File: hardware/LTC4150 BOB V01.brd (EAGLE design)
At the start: 21 parts, among them U1 LTC4150

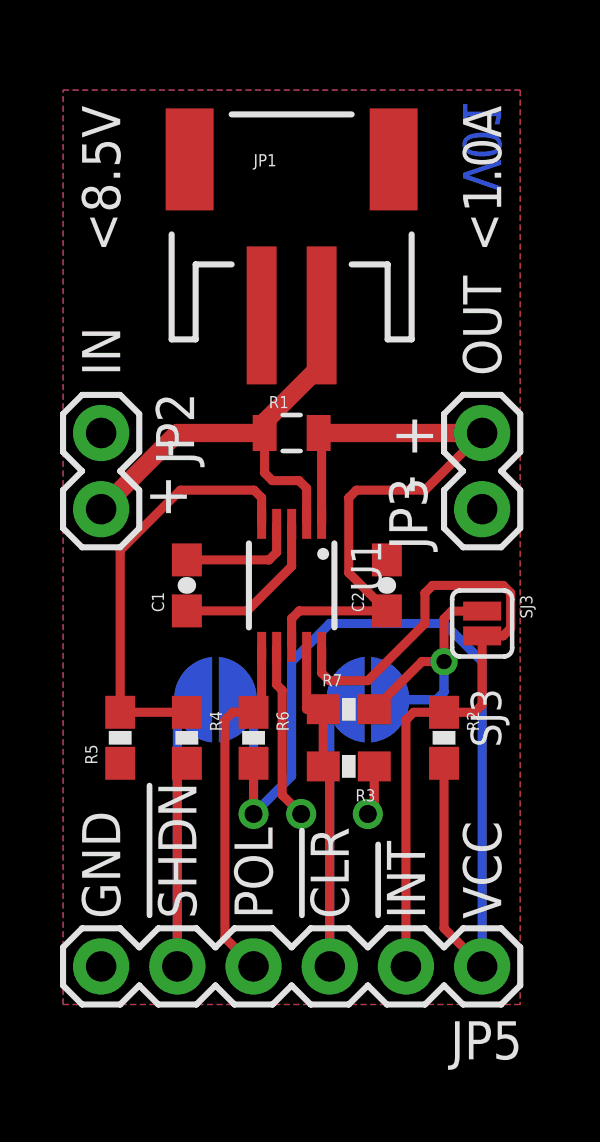
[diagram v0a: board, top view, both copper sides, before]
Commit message: Ready for proto?
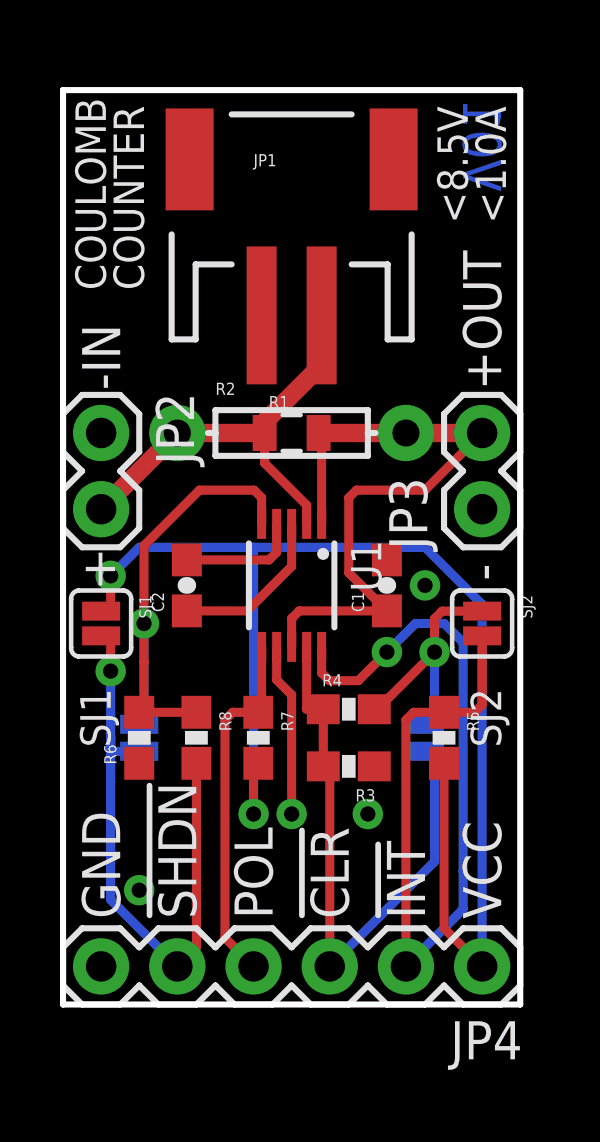
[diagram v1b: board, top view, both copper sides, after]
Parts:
- added R8: 75K, SparkFun-Passives:0603-RES
- added SJ4: (no value), mike-temp:SJ_2S-NO
- LOGO1: value LOGO-SFESK -> OSHW-LOGOS; device SparkFun-Aesthetics:SFE-LOGO-FLAME -> SparkFun-Aesthetics:OSHW-LOGO-S
- LOGO2: value OSHW-LOGOS -> LOGO-SFENW2; device SparkFun-Aesthetics:OSHW-LOGO-S -> SparkFun-Aesthetics:SFE-NEW-WEB
- LOGO3: value LOGO-SFENW2 -> LOGO-SFESK; device SparkFun-Aesthetics:SFE-NEW-WEB -> SparkFun-Aesthetics:SFE-LOGO-FLAME
- R2: value 3K -> DNP; device SparkFun-Passives:0603-RES -> SparkFun-Passives:AXIAL-0.3
- R5, R7: value 75K -> 3K
- R6: value 3K -> 75K
- SJ1: device mike-temp:SJ_ROUND -> mike-temp:SJ_2S
- SJ2: device mike-temp:SJ_ROUND -> SparkFun-Passives:SJ_2S
- SJ3: device SparkFun-Passives:SJ_2S -> mike-temp:SJ_2S-NO
- moved LOGO2 15.6 mm to (8.26, 14.0)
- moved LOGO3 12.7 mm to (8.89, 26.7)
- moved R2 11.4 mm to (7.62, 19.1), turned to 0 degrees
- moved R5 10.8 mm to (12.7, 8.89), turned to 270 degrees
- moved SJ1 9.25 mm to (1.27, 12.7), flipped to the top, turned to 270 degrees
- moved SJ2 9.25 mm to (14.0, 12.7), flipped to the top, turned to 270 degrees
- moved LOGO1 7.16 mm to (1.91, 28.3)
- moved C1 6.67 mm to (10.8, 14.0)
- moved C2 6.67 mm to (4.13, 14.0)
- moved R4 5.48 mm to (9.53, 9.84), turned to 0 degrees
- moved SJ3 4.26 mm to (12.1, 8.89), flipped to the bottom, turned to 90 degrees
- moved R6 3.81 mm to (2.54, 8.89), turned to 90 degrees
- moved R7 3.16 mm to (6.51, 8.89), turned to 270 degrees
- renumbered JP5 to JP4
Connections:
- net !CLR!: now also R4.1, SJ3.1; no longer R7.1, SJ1.1
- net !INT!: now also R5.1, SJ2.2; no longer R2.1, SJ3.2
- net !SHDN!: now also R8.2, SJ1.2, SJ4.2; no longer R4.2, SJ2.2
- net GND: now also C1.2, R6.1; no longer C2.2, R5.1
- net IN: now also R2.P$1
- net N$1: now also R4.2, SJ2.1, SJ3.2; no longer R7.2, SJ1.2, SJ3.1
- net N$3: now also C2.1; no longer C1.1
- net N$4: now also C2.2; no longer C1.2
- net N$9: now also R6.2, R8.1, SJ4.1; no longer R4.1, R5.2
- net OUT: now also C1.1, R2.P$2; no longer C2.1
- net POL: now also R7.1; no longer R6.1
- net VCC: now also R5.2, R7.2, SJ1.1; no longer R2.2, R6.2, SJ2.1
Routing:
- net VCC: track 36.0 -> 45.2 mm, vias 1 -> 2
- net !INT!: track 24.8 -> 32.0 mm, vias 0 -> 1
- net !SHDN!: track 16.0 -> 20.7 mm, vias 0 -> 1
- net N$9: track 14.1 -> 16.8 mm, vias 0 -> 1
- net GND: track 7.59 -> 5.78 mm, vias 2 -> 4
- net IN: track 15.3 -> 14.8 mm
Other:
- board outline added: 15.2 x 30.5 mm
- board text added: "+"
- board text added: "+OUT"
- board text added: "-"
- board text added: "-IN"
- board text added: "COULOMB"
- board text added: "COUNTER"
- board text added: "SJ4"
- board text removed: "+ -"
- board text removed: "IN"
- board text removed: "OUT"
